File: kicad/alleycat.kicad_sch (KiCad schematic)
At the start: 1 part

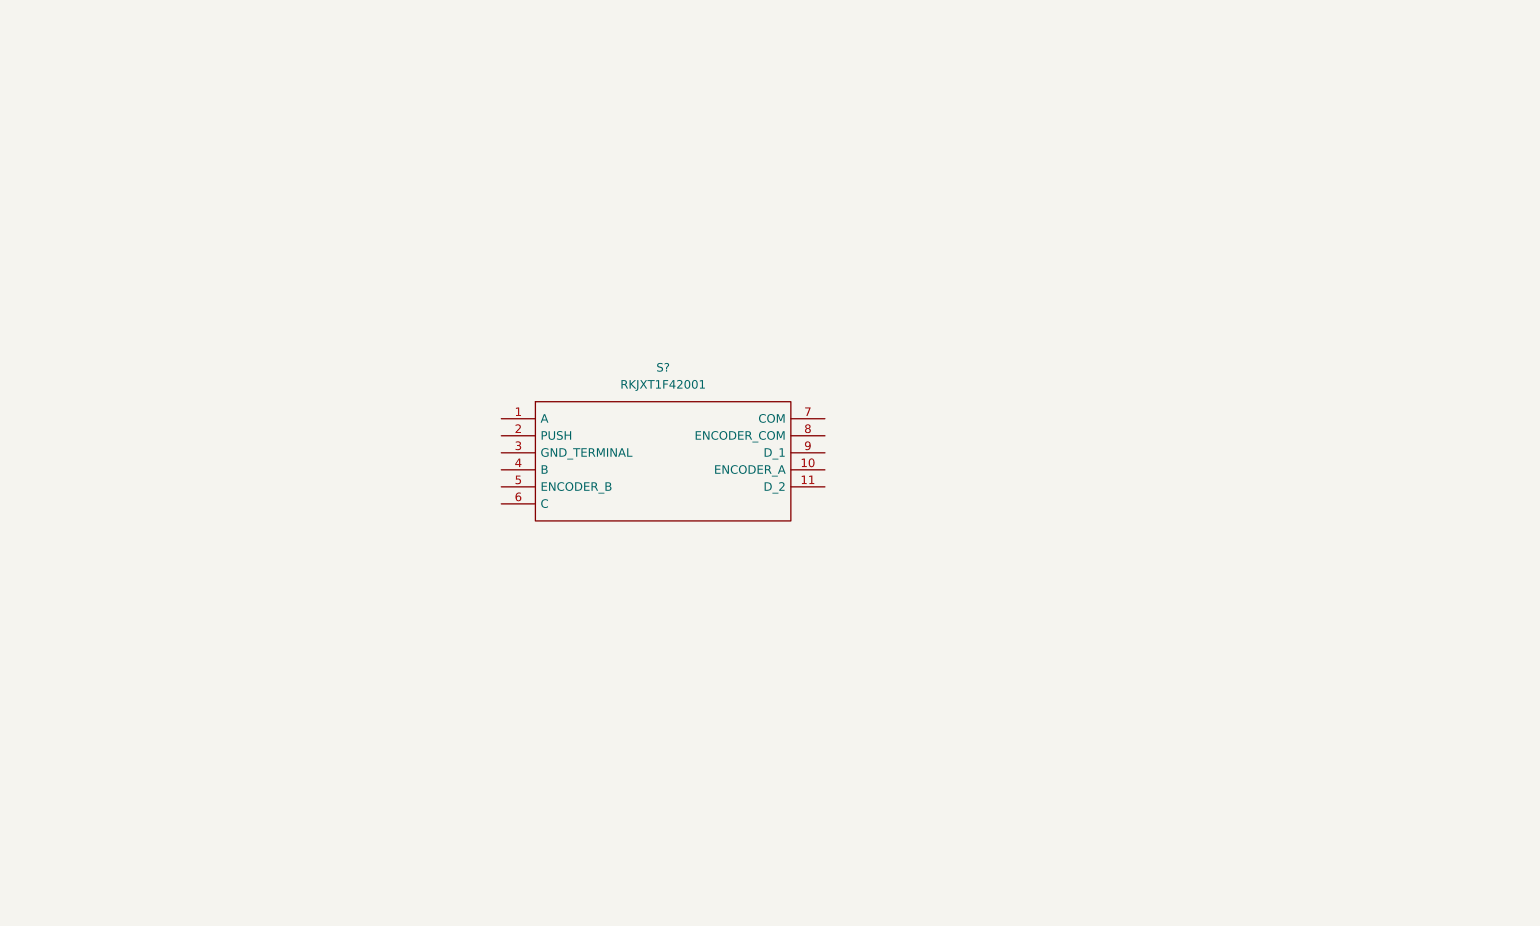
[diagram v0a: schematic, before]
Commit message: modified schematic
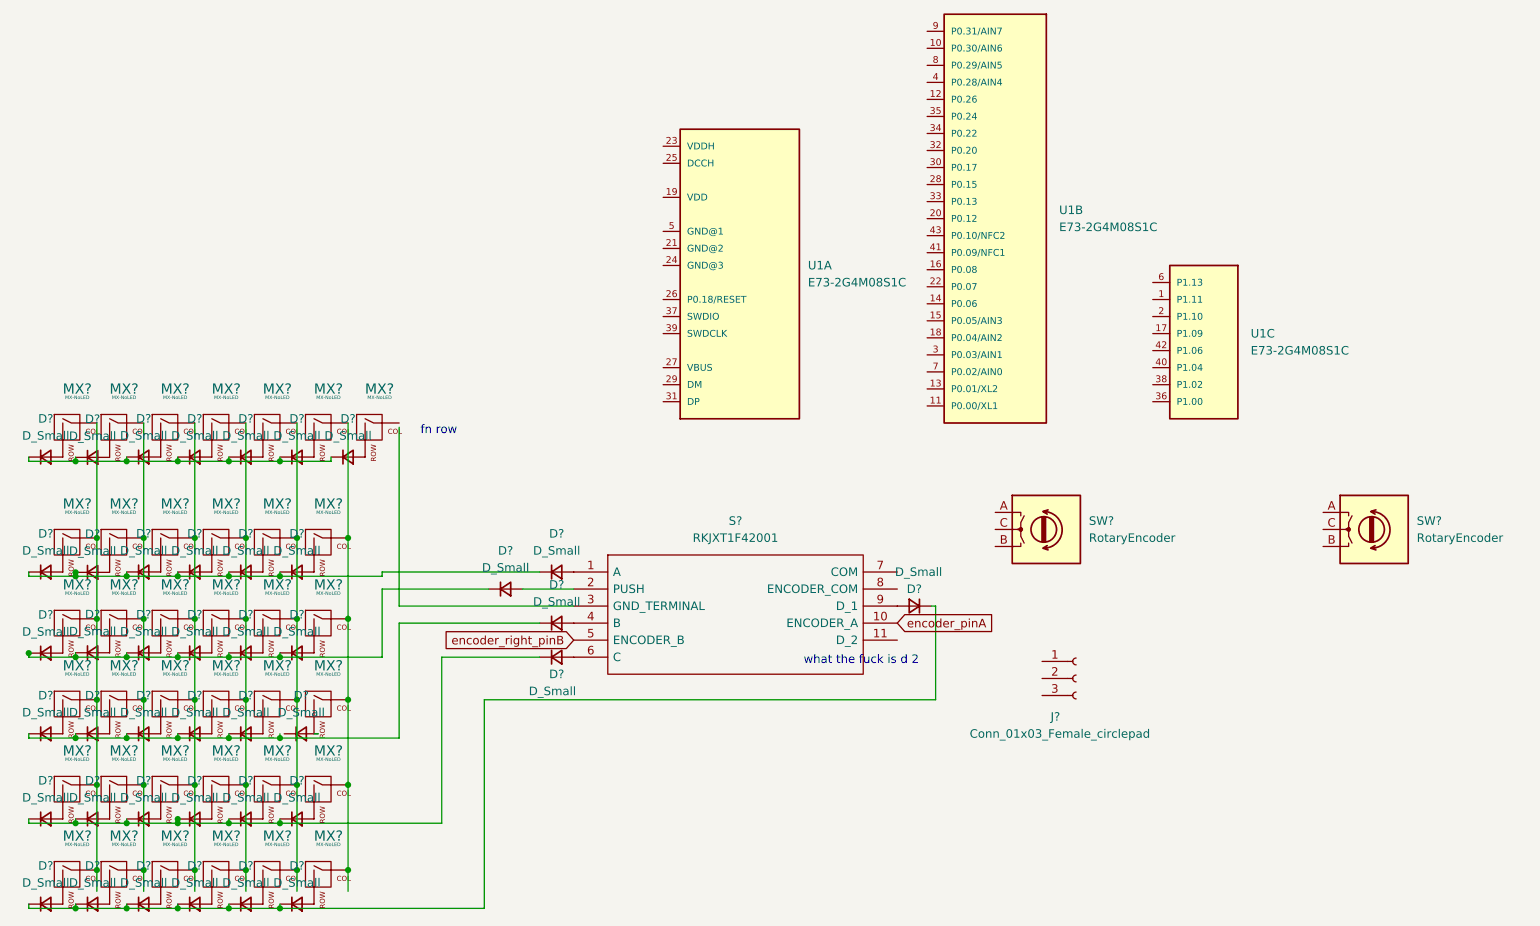
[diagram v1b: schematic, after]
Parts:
- added D? (x42): D_Small, symbol Device:D_Small
- added J?: Conn_01x03_Female_circlepad, symbol Connector:Conn_01x03_Female
- added MX? (x37): MX-NoLED, symbol MX_Alps_Hybrid:MX-NoLED
- added SW? (x2): RotaryEncoder, symbol Device:RotaryEncoder
- added U1: E73-2G4M08S1C, E73-2G4M08S1C, symbol E73-2G4M08S1C:E73-2G4M08S1C
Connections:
- net at S?.1 (A): now also D?.2 (A)
- net encoder_pinA: now reaches S?.10 (ENCODER_A)
- net at S?.2 (PUSH): now also D?.2 (A)
- net at S?.4 (B): now also D?.2 (A)
- net encoder_right_pinB: now reaches S?.5 (ENCODER_B)
- net at S?.6 (C): now also D?.2 (A)
- net at S?.9 (D_1): now also D?.2 (A)
- new net: D?.1 (K), D?.1 (K), D?.1 (K), D?.1 (K), D?.1 (K), D?.1 (K) (x3)
- new net: D?.2 (A), MX?.2 (ROW) (x30)
- new net: MX?.1 (COL), MX?.1 (COL), MX?.1 (COL), MX?.1 (COL), MX?.1 (COL), MX?.1 (COL) (x6)
- new net: D?.1 (K), D?.1 (K), D?.1 (K), D?.1 (K), D?.1 (K)
- new net: D?.1 (K), D?.1 (K), D?.1 (K), D?.1 (K), D?.1 (K), D?.1 (K), D?.1 (K) (x2)
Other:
- note added: "fn row"
- note added: "what the fuck is d 2"
- moved on the sheet: S?
